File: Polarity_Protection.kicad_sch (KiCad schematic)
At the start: 7 parts, among them J1 IN+, J2 IN-, Q1 BSS214NW

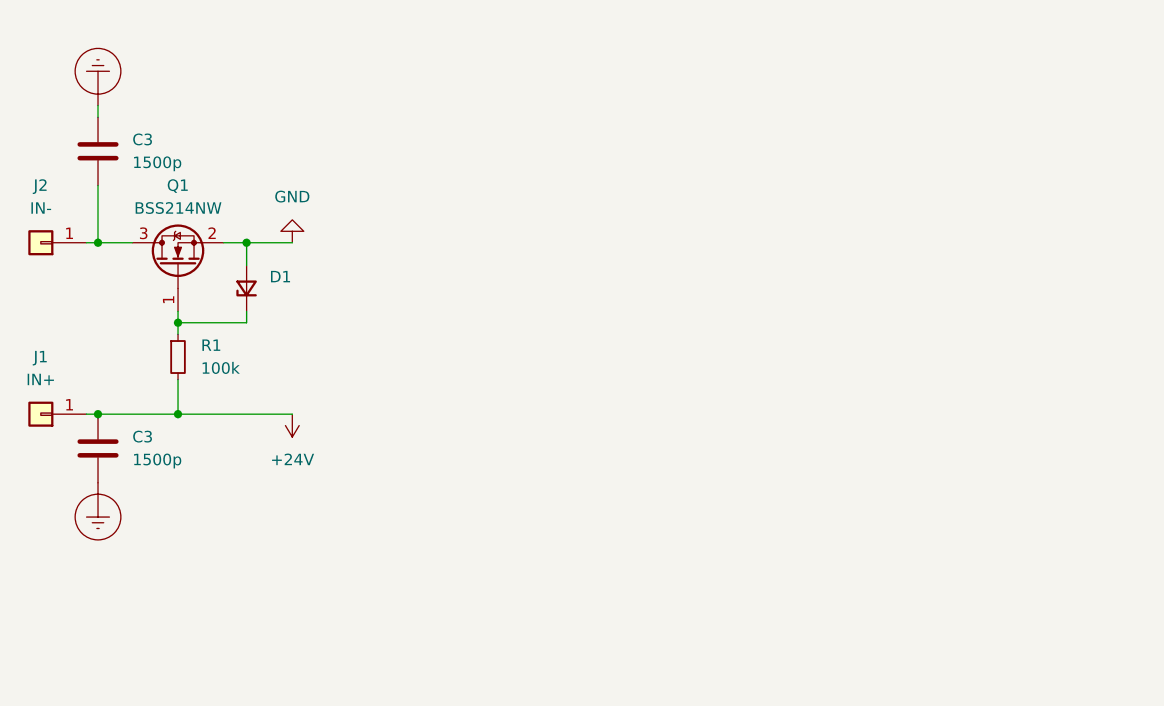
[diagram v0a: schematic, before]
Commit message: Отчётная версия
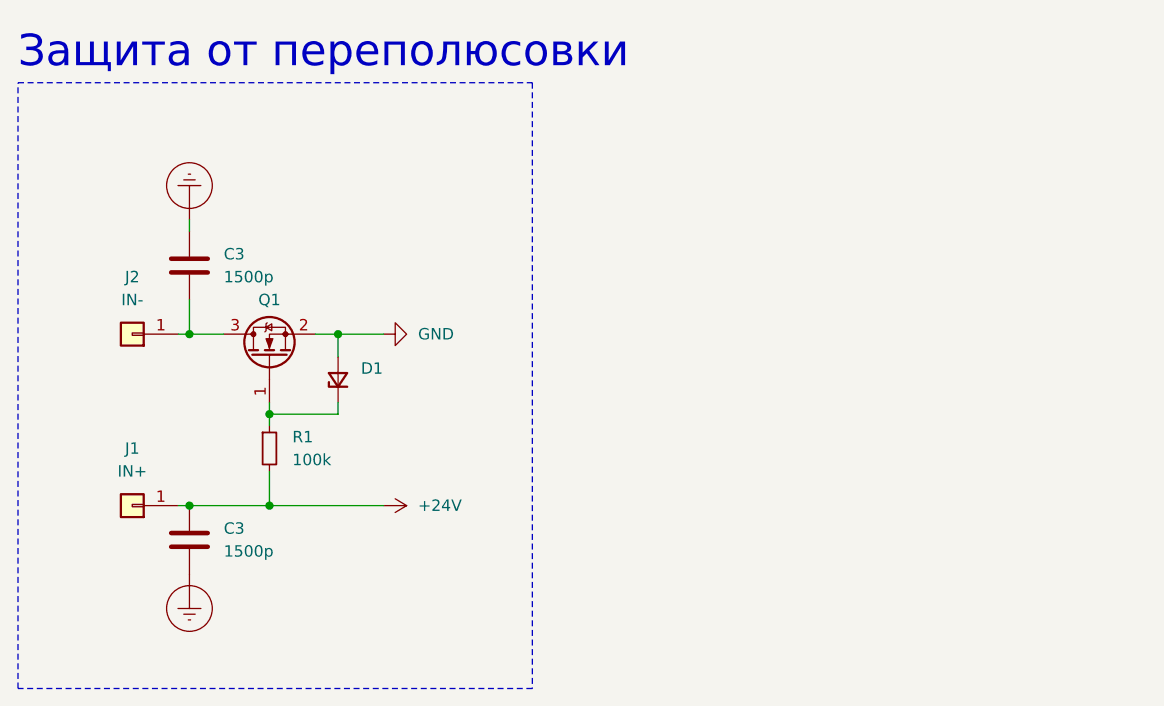
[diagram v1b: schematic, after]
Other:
- note added: "Защита от переполюсовки"
- company: (none) -> Московский Политех
- moved on the sheet: C3, D1, J1, J2, Q1, R1
